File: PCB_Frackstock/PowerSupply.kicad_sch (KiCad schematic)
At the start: 25 parts, among them J2 105450-0101, U12 SPX3819M5-L-3-3/TR, U14 1043, U3 MCP73871-2CC, U4 TPS61222DCK

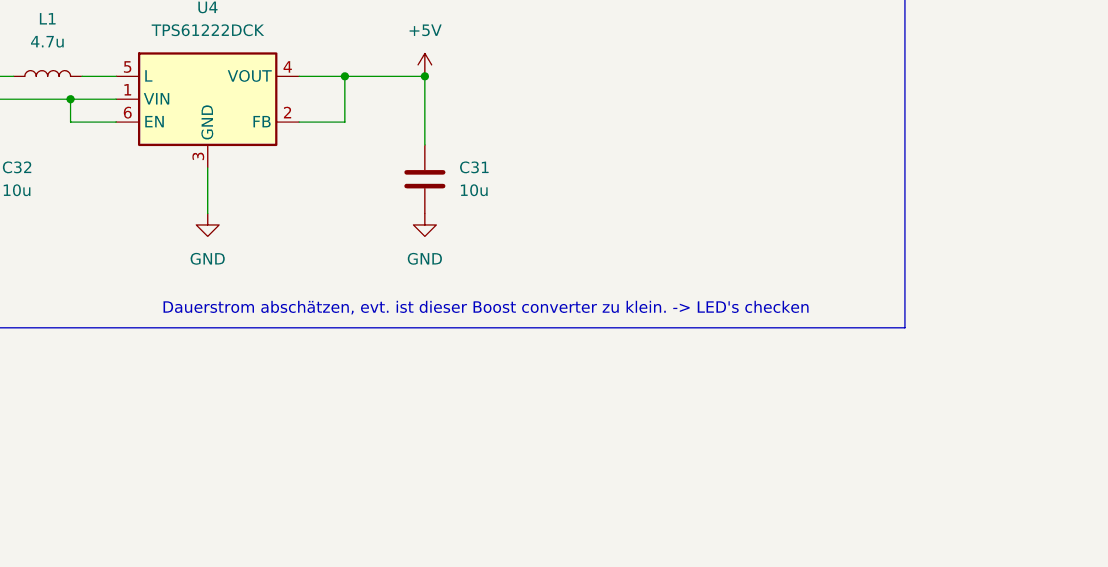
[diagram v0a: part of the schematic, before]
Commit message: Schema fertig
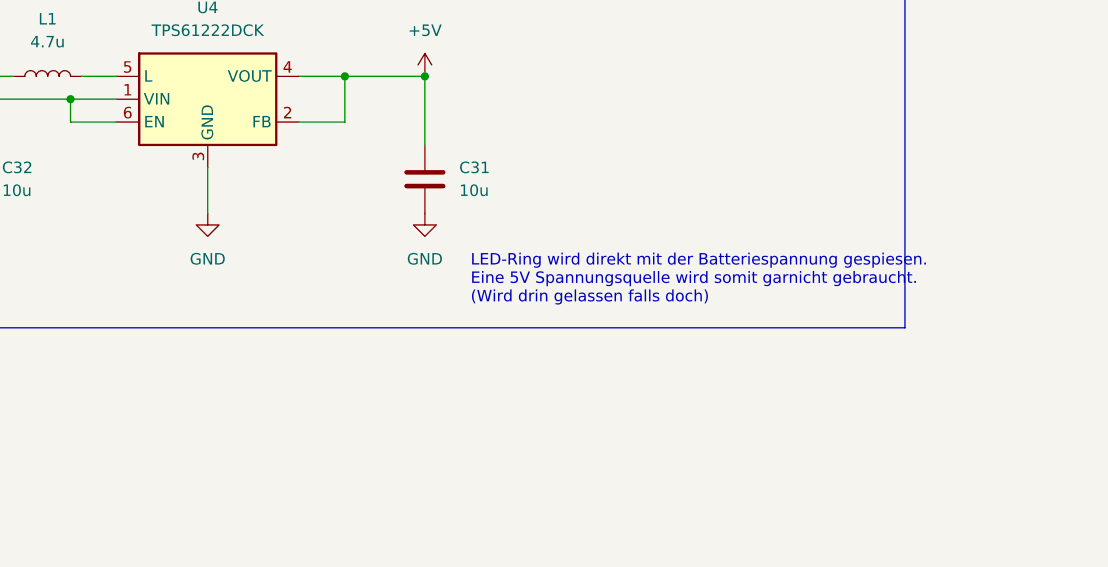
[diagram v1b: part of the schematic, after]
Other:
- note added: "LED-Ring wird direkt mit der Batteriespannung gespiesen. Eine 5V Spannungsquelle wird somit garnicht gebraucht. (Wird drin gelassen falls doch)"
- note removed: "Dauerstrom abschätzen, evt. ist dieser Boost converter zu klein. -> LED's checken"
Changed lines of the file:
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@@
     (effects (font (size 1.27 1.27)) (justify left bottom))
   )
-  (text "Dauerstrom abschätzen, evt. ist dieser Boost converter zu klein. -> LED's checken"
-    (at 193.04 158.75 0)
+  (text "LED-Ring wird direkt mit der Batteriespannung gespiesen.\nEine 5V Spannungsquelle wird somit garnicht gebraucht.\n(Wird drin gelassen falls doch)\n"
+    (at 227.33 157.48 0)
     (effects (font (size 1.27 1.27)) (justify left bottom))
   )
